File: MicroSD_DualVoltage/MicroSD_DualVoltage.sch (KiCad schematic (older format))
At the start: 18 parts, among them J1 Conn_01x08, J3 Micro_SD_Card_Det, U1 AP7365, U2 TXB0104PW

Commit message: Schematic PDF and 3D Renders added
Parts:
- U1: symbol U.FL-R-SMT(01):AP7365 -> MicroSD_DualVoltage-rescue:AP7365-U.FL-R-SMT(01)
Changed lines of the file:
@@
 $EndComp
 $Comp
-L U.FL-R-SMT(01):AP7365 U1
+L MicroSD_DualVoltage-rescue:AP7365-U.FL-R-SMT(01) U1
 U 1 1 5DB62551
 P 4850 5950

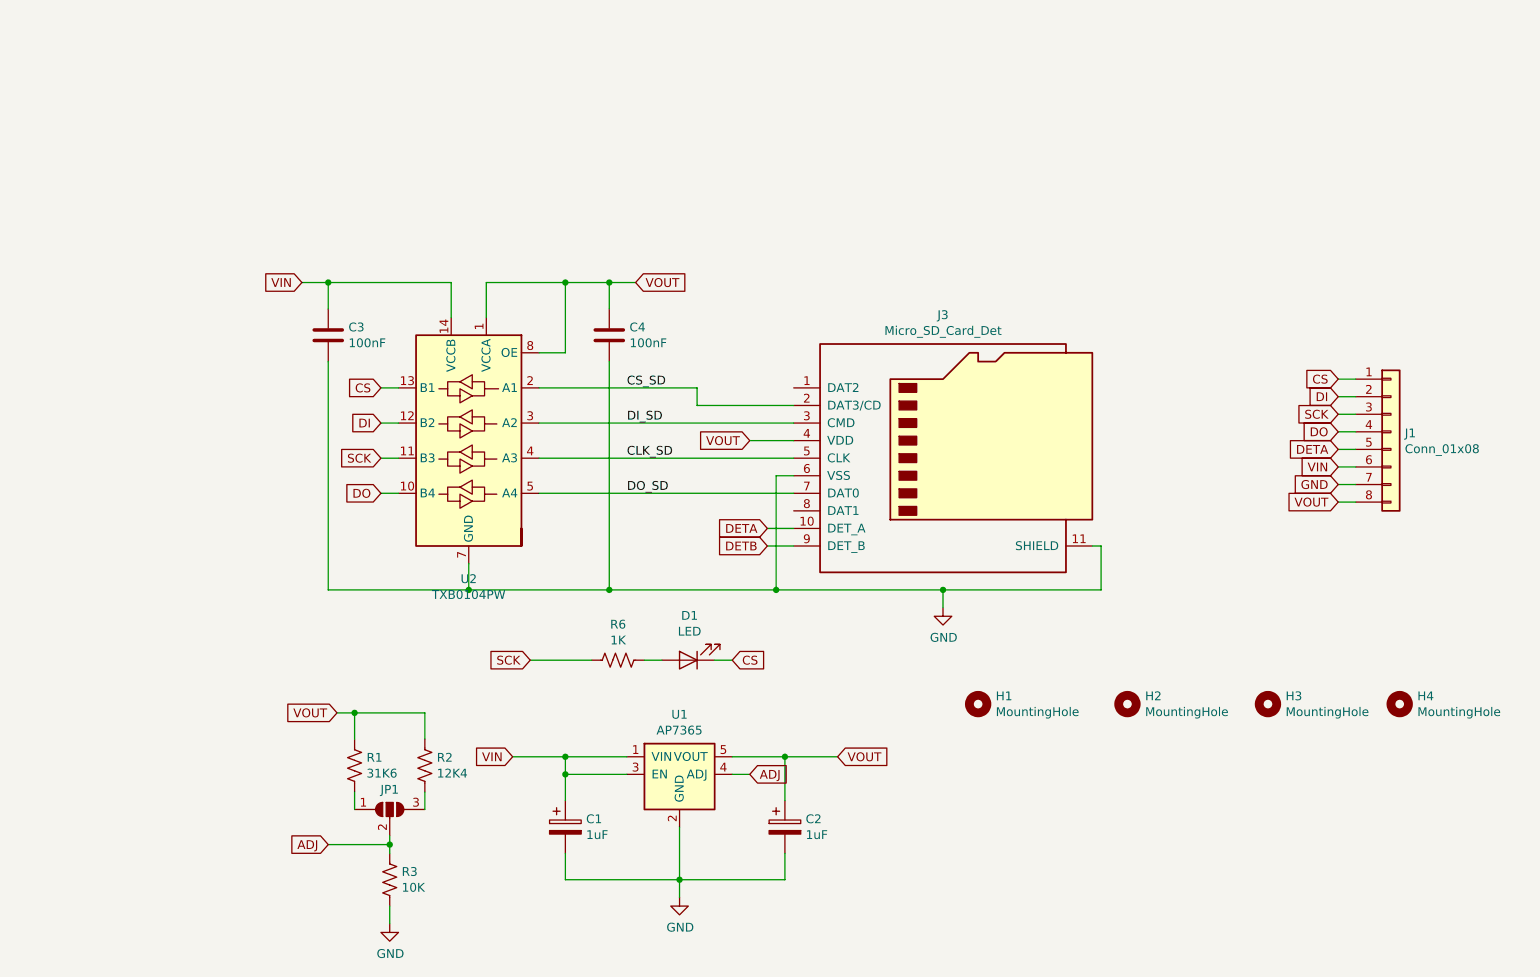
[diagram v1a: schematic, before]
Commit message: Board Redesign
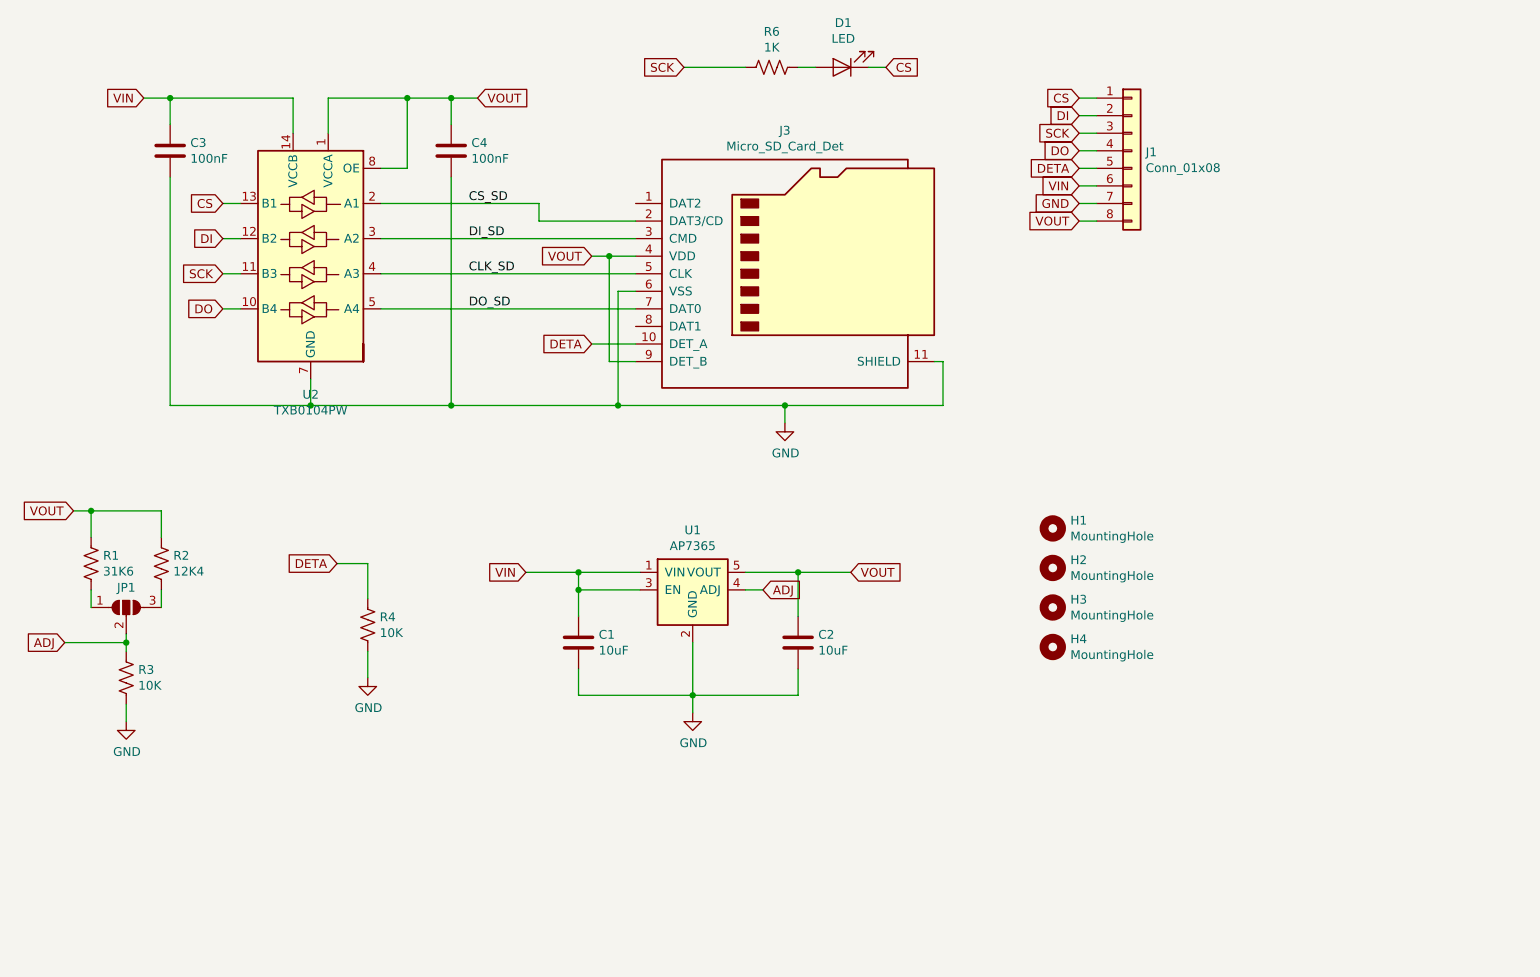
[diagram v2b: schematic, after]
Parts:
- removed C1, C2: 1uF, Capacitor_SMD:C_0603_1608Metric, symbol Device:CP
- added C1, C2: 10uF, Capacitor_SMD:C_0805_2012Metric, symbol Device:C
- added R4: 10K, Resistor_SMD:R_0603_1608Metric, symbol Device:R_US
- H1, H2, H3, H4: footprint MountingHole:MountingHole_2.7mm_M2.5_ISO14580_Pad -> SirBoardLibrary:MountingHole_M2.5_SirBoard
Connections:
- net DETB is gone; now on net VOUT: J3.9 (DET_B)
- net DETA: now also R4.1
- net GND: now also C1.2, C2.2, R4.2
- net VIN: now also C1.1
- net VOUT: now also C2.1
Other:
- moved on the sheet: C3, C4, D1, H1, J1, J3, JP1, R1, R2, R3, R6, U1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
